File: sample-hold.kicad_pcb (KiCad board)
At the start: 2 copper layers, 65.7 x 89.7 mm, 91 parts, among them J1 Conn_02x05_Odd_Even, J10 Conn_01x03_Socket, J11 Conn_01x03_Pin, J12 Conn_01x03_Socket, J2 AudioJack2_SwitchT, J3 AudioJack2_SwitchT, J4 AudioJack2_SwitchT, J5 AudioJack2_SwitchT, J6 AudioJack2_SwitchT, J7 Conn_01x03_Pin, J8 Conn_01x03_Socket, J9 Conn_01x03_Pin, Q1 BC547C, Q2 BCM847, Q3 MMBF4393, SW1 ON-ON-ON, U1 TL074, U2 TL074

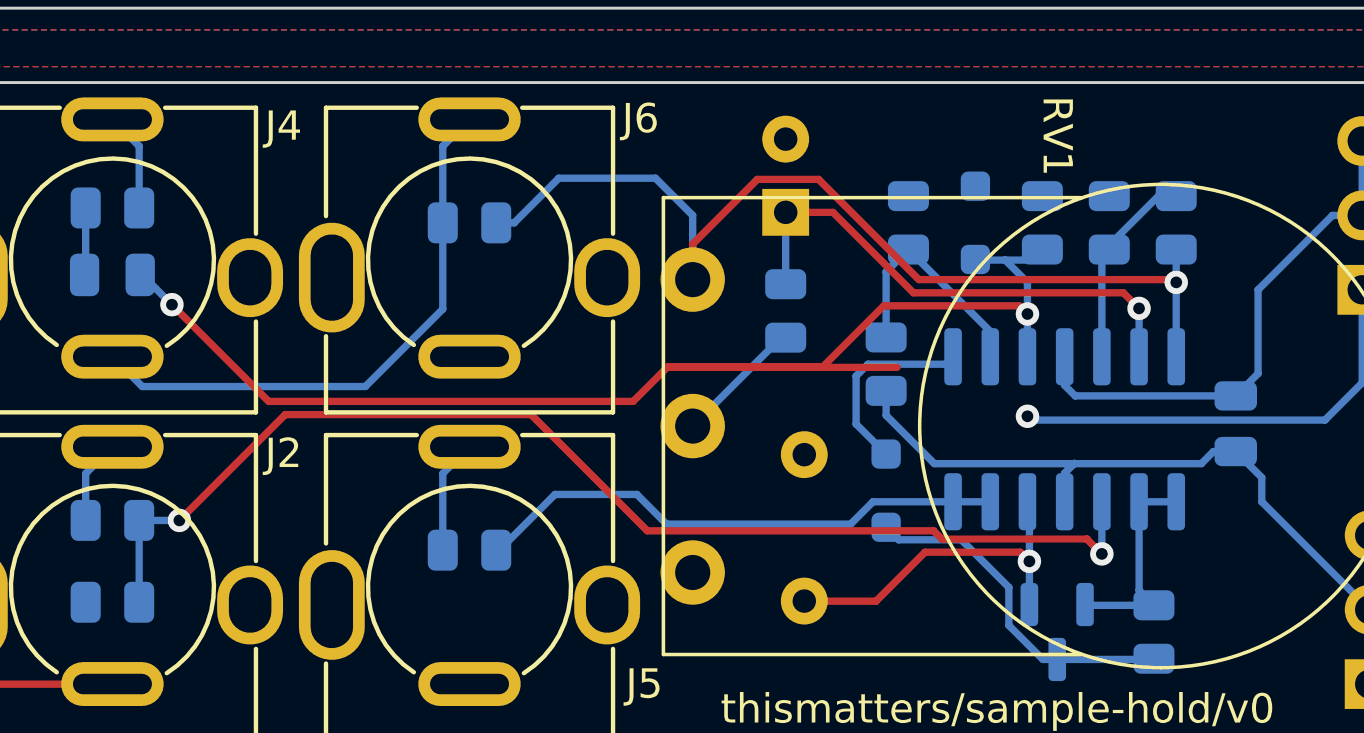
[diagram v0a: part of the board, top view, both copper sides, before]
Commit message: little routing cleanup
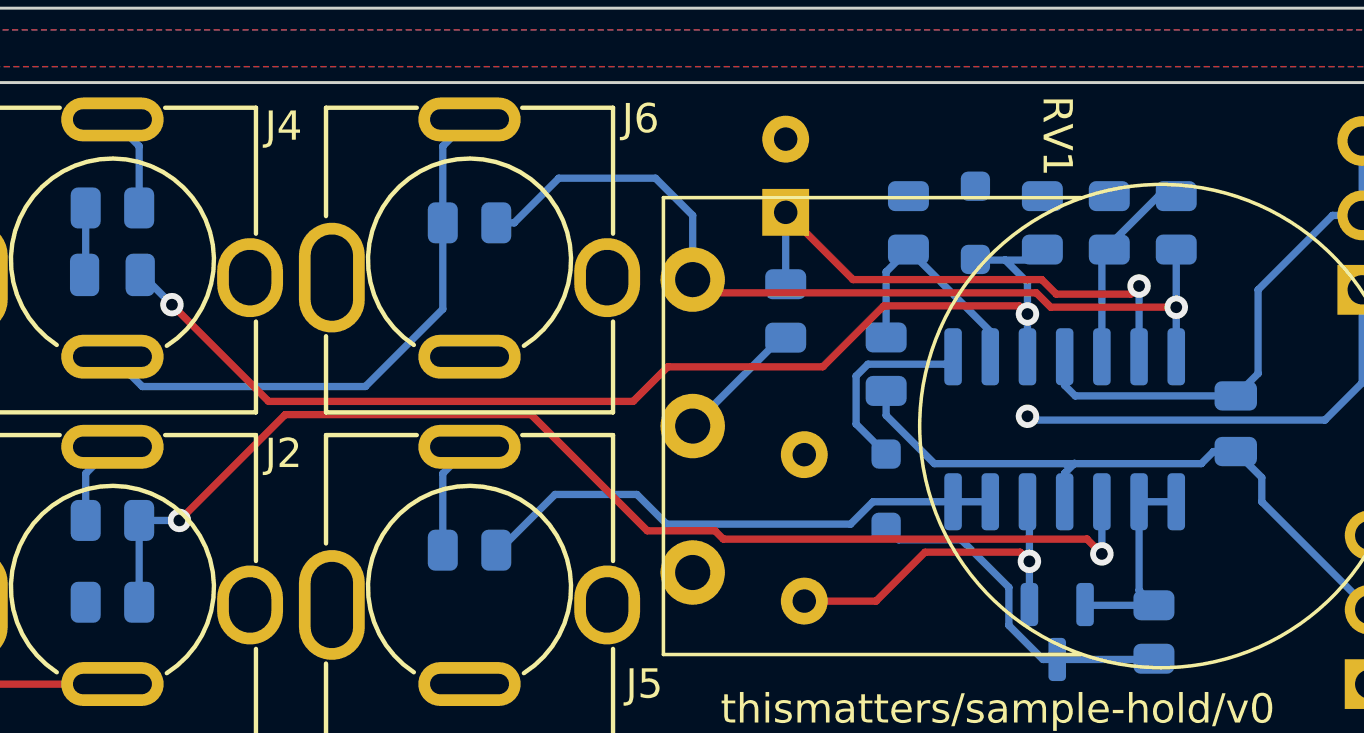
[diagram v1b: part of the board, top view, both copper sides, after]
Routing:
- net Net-(D3-K): track 46.9 -> 39.0 mm
- net Net-(R35-Pad2): track 33.8 -> 30.6 mm
- net Net-(U2D--): track 17.5 -> 18.2 mm
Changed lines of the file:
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@@
   (segment (start 101.5795 86.571) (end 101.854 86.8455) (width 0.25) (layer "F.Cu") (net 30))
   (segment (start 89.555 88.666) (end 89.575 88.646) (width 0.25) (layer "F.Cu") (net 30))
-  (segment (start 89.555 88.666) (end 97.404 88.666) (width 0.25) (layer "F.Cu") (net 30))
   (segment (start 72.644 86.527) (end 75.946 89.829) (width 0.25) (layer "F.Cu") (net 30))
   (via (at 101.854 86.8455) (size 0.8) (drill 0.4) (layers "F.Cu" "B.Cu") (net 30))
@@
   (segment (start 85.723 93.006) (end 83.82 94.909) (width 0.25) (layer "B.Cu") (net 46))
   (segment (start 96.5799 93.255) (end 95.8149 94.02) (width 0.25) (layer "B.Cu") (net 46))
-  (segment (start 98.933 94.528) (end 103.886 94.528) (width 0.25) (layer "F.Cu") (net 47))
-  (segment (start 76.512 90.279) (end 84.905 90.279) (width 0.25) (layer "F.Cu") (net 47))
-  (segment (start 98.651 94.246) (end 98.933 94.528) (width 0.25) (layer "F.Cu") (net 47))
-  (segment (start 88.872 94.246) (end 98.651 94.246) (width 0.25) (layer "F.Cu") (net 47))
-  (segment (start 103.886 94.528) (end 104.394 95.036) (width 0.25) (layer "F.Cu") (net 47))
-  (segment (start 84.905 90.279) (end 88.872 94.246) (width 0.25) (layer "F.Cu") (net 47))
-  (segment (start 72.898 93.893) (end 76.512 90.279) (width 0.25) (layer "F.Cu") (net 47))
+  (segment (start 76.512 90.279) (end 72.898 93.893) (width 0.25) (layer "F.Cu") (net 47))
+  (segment (start 91.468 94.528) (end 91.186 94.246) (width 0.25) (layer "F.Cu") (net 47))
+  (segment (start 84.905 90.279) (end 76.512 90.279) (width 0.25) (layer "F.Cu") (net 47))
+  (segment (start 88.872 94.246) (end 84.905 90.279) (width 0.25) (layer "F.Cu") (net 47))
+  (segment (start 104.394 95.036) (end 103.886 94.528) (width 0.25) (layer "F.Cu") (net 47))
+  (segment (start 103.886 94.528) (end 91.468 94.528) (width 0.25) (layer "F.Cu") (net 47))
+  (segment (start 91.186 94.246) (end 88.872 94.246) (width 0.25) (layer "F.Cu") (net 47))
   (via (at 72.898 93.893) (size 0.8) (drill 0.4) (layers "F.Cu" "B.Cu") (net 47))
   (via (at 104.394 95.036) (size 0.8) (drill 0.4) (layers "F.Cu" "B.Cu") (net 47))
@@
   (segment (start 58.42 85.003) (end 60.96 85.003) (width 0.25) (layer "B.Cu") (net 49))
   (segment (start 55.88 82.463) (end 58.42 85.003) (width 0.25) (layer "B.Cu") (net 49))
-  (segment (start 95.212604 83.374113) (end 97.959491 86.121) (width 0.25) (layer "F.Cu") (net 50))
-  (segment (start 97.959491 86.121) (end 105.131 86.121) (width 0.25) (layer "F.Cu") (net 50))
-  (segment (start 93.599 83.374113) (end 95.212604 83.374113) (width 0.25) (layer "F.Cu") (net 50))
-  (segment (start 105.131 86.121) (end 105.664 86.654) (width 0.25) (layer "F.Cu") (net 50))
-  (via (at 105.664 86.654) (size 0.8) (drill 0.4) (layers "F.Cu" "B.Cu") (net 50))
-  (segment (start 105.664 86.654) (end 105.664 88.305) (width 0.25) (layer "B.Cu") (net 50))
+  (segment (start 102.340701 85.6705) (end 102.834201 86.164) (width 0.25) (layer "F.Cu") (net 50))
+  (segment (start 93.599 83.374113) (end 95.895888 85.671) (width 0.25) (layer "F.Cu") (net 50))
+  (segment (start 101.854 85.671) (end 101.8545 85.6705) (width 0.25) (layer "F.Cu") (net 50))
+  (segment (start 102.834201 86.164) (end 105.3895 86.164) (width 0.25) (layer "F.Cu") (net 50))
+  (segment (start 101.8545 85.6705) (end 102.340701 85.6705) (width 0.25) (layer "F.Cu") (net 50))
+  (segment (start 105.3895 86.164) (end 105.664 85.8895) (width 0.25) (layer "F.Cu") (net 50))
+  (segment (start 95.895888 85.671) (end 101.854 85.671) (width 0.25) (layer "F.Cu") (net 50))
+  (via (at 105.664 85.8895) (size 0.8) (drill 0.4) (layers "F.Cu" "B.Cu") (net 50))
   (segment (start 93.599 83.374113) (end 93.599 85.8285) (width 0.25) (layer "B.Cu") (net 50))
+  (segment (start 105.664 85.8895) (end 105.664 88.305) (width 0.25) (layer "B.Cu") (net 50))
   (segment (start 90.424 90.671) (end 93.4415 87.6535) (width 0.25) (layer "B.Cu") (net 52))
-  (segment (start 93.4415 87.6535) (end 93.599 87.6535) (width 0.25) (layer "B.Cu") (net 52))
   (segment (start 104.394 88.305) (end 104.394 84.8995) (width 0.25) (layer "B.Cu") (net 53))
   (segment (start 106.3225 82.8205) (end 106.934 82.8205) (width 0.25) (layer "B.Cu") (net 53))
   (segment (start 104.648 84.495) (end 106.3225 82.8205) (width 0.25) (layer "B.Cu") (net 53))
-  (segment (start 92.629887 82.249113) (end 94.724 82.249113) (width 0.25) (layer "F.Cu") (net 55))
-  (segment (start 106.807 85.765) (end 106.934 85.765) (width 0.25) (layer "F.Cu") (net 55))
-  (segment (start 90.424 84.455) (end 92.629887 82.249113) (width 0.25) (layer "F.Cu") (net 55))
-  (segment (start 106.713 85.671) (end 106.807 85.765) (width 0.25) (layer "F.Cu") (net 55))
-  (segment (start 98.145887 85.671) (end 106.713 85.671) (width 0.25) (layer "F.Cu") (net 55))
-  (segment (start 94.724 82.249113) (end 98.145887 85.671) (width 0.25) (layer "F.Cu") (net 55))
-  (segment (start 90.424 85.671) (end 90.424 84.455) (width 0.25) (layer "F.Cu") (net 55))
-  (via (at 106.934 85.765) (size 0.8) (drill 0.4) (layers "F.Cu" "B.Cu") (net 55))
+  (segment (start 102.154305 86.1205) (end 90.8735 86.1205) (width 0.25) (layer "F.Cu") (net 55))
+  (segment (start 90.8735 86.1205) (end 90.424 85.671) (width 0.25) (layer "F.Cu") (net 55))
+  (segment (start 106.934 86.614) (end 102.647805 86.614) (width 0.25) (layer "F.Cu") (net 55))
+  (segment (start 102.647805 86.614) (end 102.154305 86.1205) (width 0.25) (layer "F.Cu") (net 55))
+  (via (at 106.934 86.614) (size 0.8) (drill 0.4) (layers "F.Cu" "B.Cu") (net 55))
+  (segment (start 106.934 84.6455) (end 106.934 86.614) (width 0.25) (layer "B.Cu") (net 55))
   (segment (start 83.7165 83.733) (end 84.328 83.733) (width 0.25) (layer "B.Cu") (net 55))
-  (segment (start 106.934 84.6455) (end 106.934 85.765) (width 0.25) (layer "B.Cu") (net 55))
-  (segment (start 106.934 85.765) (end 106.934 88.305) (width 0.25) (layer "B.Cu") (net 55))
+  (segment (start 106.934 86.614) (end 106.934 88.305) (width 0.25) (layer "B.Cu") (net 55))
   (segment (start 84.328 83.733) (end 85.852 82.209) (width 0.25) (layer "B.Cu") (net 55))
   (segment (start 85.852 82.209) (end 89.154 82.209) (width 0.25) (layer "B.Cu") (net 55))
